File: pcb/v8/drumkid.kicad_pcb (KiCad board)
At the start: 2 copper layers, 90 x 140 mm, 57 parts, among them J1 DIN-5_180degree, J2 DIN-5_180degree, J3 Conn_01x15, J4 Conn_01x15, J9 AudioJack3_Ground_Switch, SW1 SW_Push, SW2 SW_Push, SW3 SW_Push, SW4 SW_Push, SW5 SW_Push, SW6 SW_Push, SW7 SW_SPDT, SW8 SW_SPDT, U1 6N138

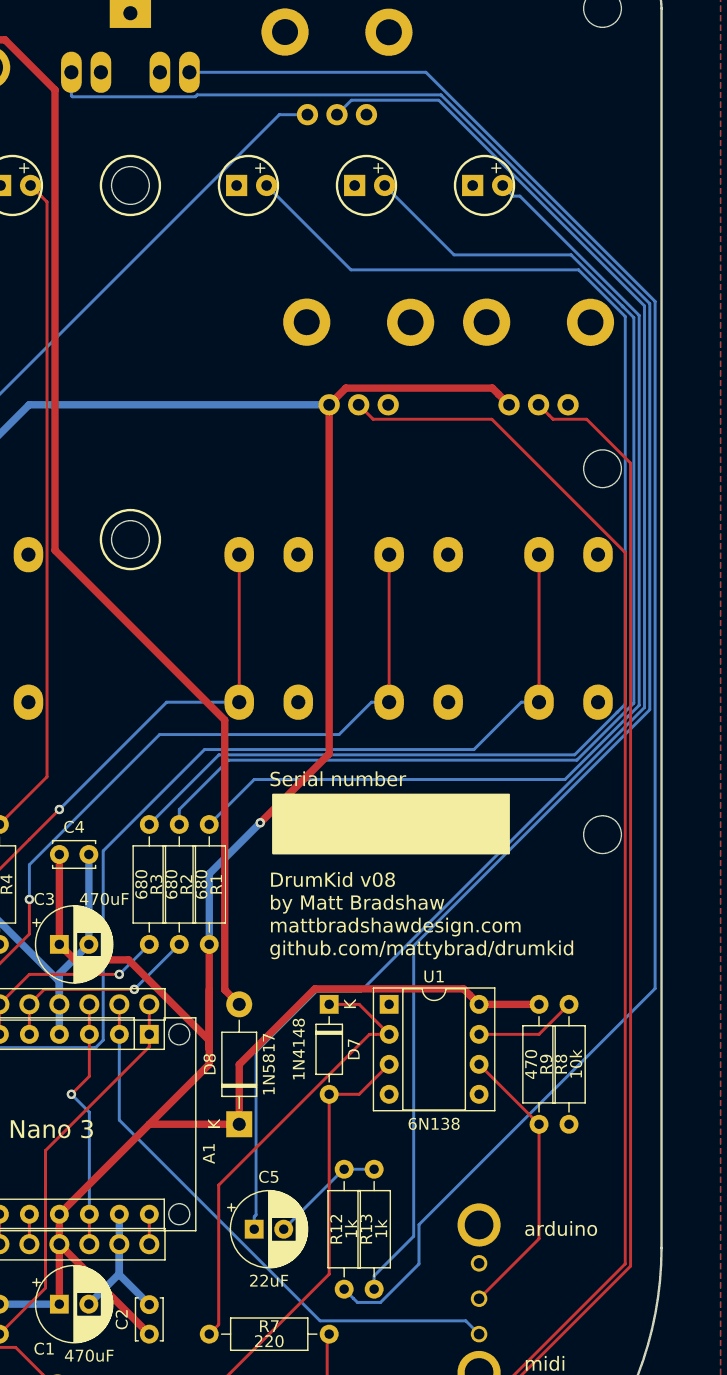
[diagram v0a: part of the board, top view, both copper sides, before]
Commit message: v8 gerbers done
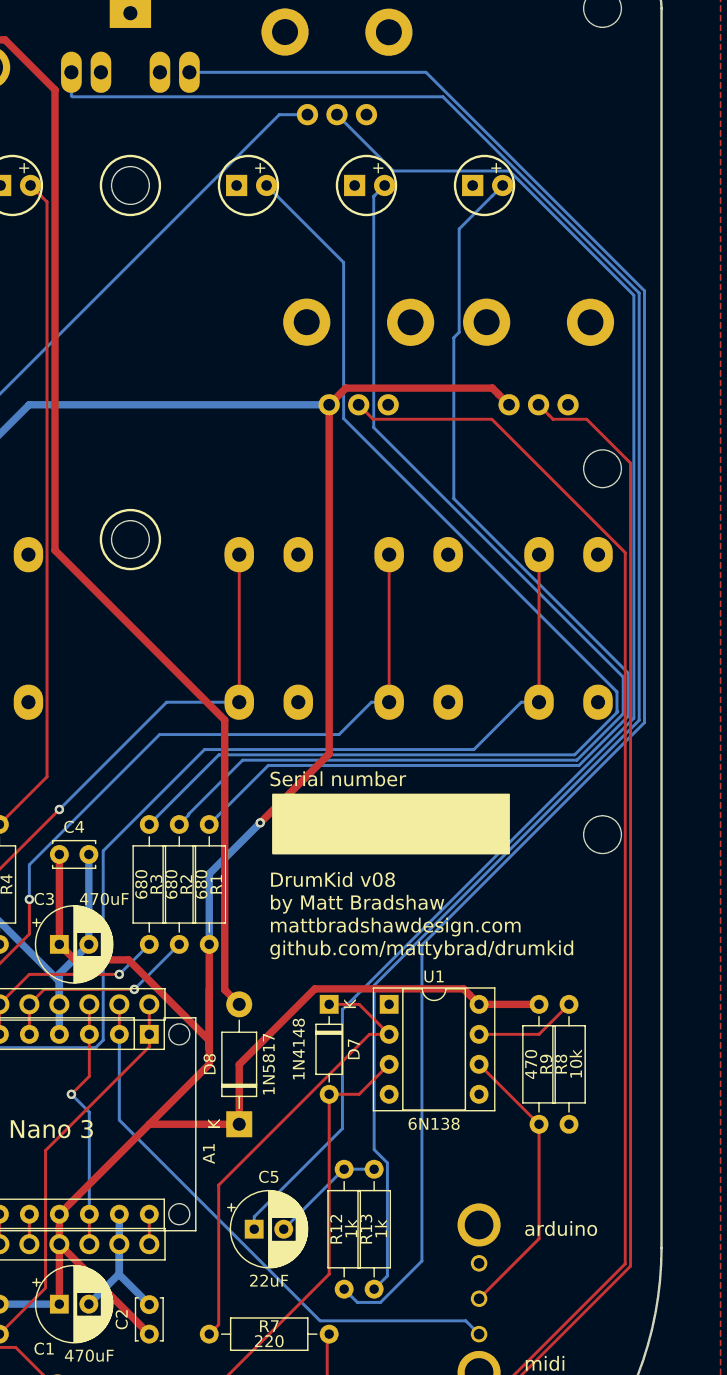
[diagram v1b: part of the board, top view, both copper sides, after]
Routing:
- net Net-(D3-Pad2): track 112.5 -> 100.6 mm
- net Net-(D2-Pad2): track 102.1 -> 95.4 mm
- net Net-(C5-Pad1): track 127.9 -> 123.9 mm
- net Net-(D1-Pad2): track 89.8 -> 92.1 mm
- net Net-(J9-PadT): track 145.5 -> 145.0 mm
